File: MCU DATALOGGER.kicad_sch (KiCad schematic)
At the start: 26 parts, among them U1 24LC1025, U2 24LC1025, U3 ATMEGA328P-AU, U4 DS1337S_, Y1 16MHz, Y2 32.768 KHz

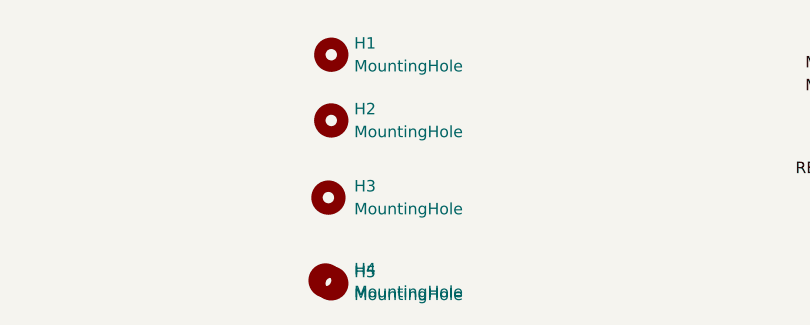
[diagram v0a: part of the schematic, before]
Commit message: done the placing
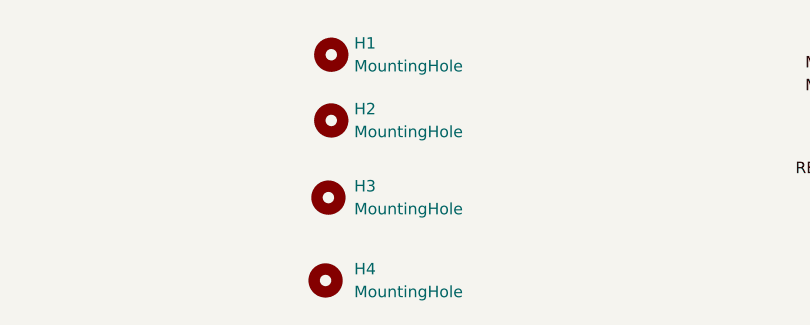
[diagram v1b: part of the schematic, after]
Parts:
- removed H5: MountingHole, MountingHole:MountingHole_2.1mm, symbol Mechanical:MountingHole
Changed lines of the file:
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@@
-	)
-	(symbol
-		(lib_id "Mechanical:MountingHole")
-		(at 152.4 168.5925 0)
-		(unit 1)
-		(exclude_from_sim no)
-		(in_bom no)
-		(on_board yes)
-		(dnp no)
-		(fields_autoplaced yes)
-		(property "Reference" "H5"
-			(at 154.94 167.3224 0)
-			(effects
-				(font
-					(size 1.27 1.27)
-				)
-				(justify left)
-			)
-		)
-		(property "Value" "MountingHole"
-			(at 154.94 169.8624 0)
-			(effects
-				(font
-					(size 1.27 1.27)
-				)
-				(justify left)
-			)
-		)
-		(property "Footprint" "MountingHole:MountingHole_2.1mm"
-			(at 152.4 168.5925 0)
-			(effects
-				(font
-					(size 1.27 1.27)
-				)
-				(hide yes)
-			)
-		)
-		(property "Datasheet" "~"
-			(at 152.4 168.5925 0)
-			(effects
-				(font
-					(size 1.27 1.27)
-				)
-				(hide yes)
-			)
-		)
-		(property "Description" "Mounting Hole without connection"
-			(at 152.4 168.5925 0)
-			(effects
-				(font
-					(size 1.27 1.27)
-				)
-				(hide yes)
-			)
-		)
-		(instances
-			(project ""
-				(path "/dc0dacd0-94d8-4dc0-9d43-b772496c3eb2"
-					(reference "H5")
-					(unit 1)
-				)
-			)
-		)
 	)
 	(symbol
